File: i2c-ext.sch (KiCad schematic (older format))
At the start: 5 parts, among them J1101 SMBUS, U1101 TCA9802

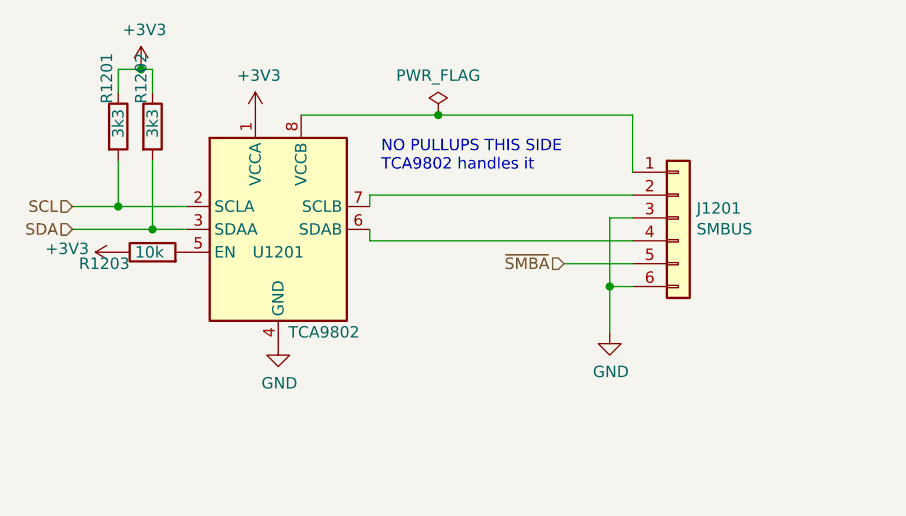
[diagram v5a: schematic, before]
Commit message: MB: add caps suggested in review
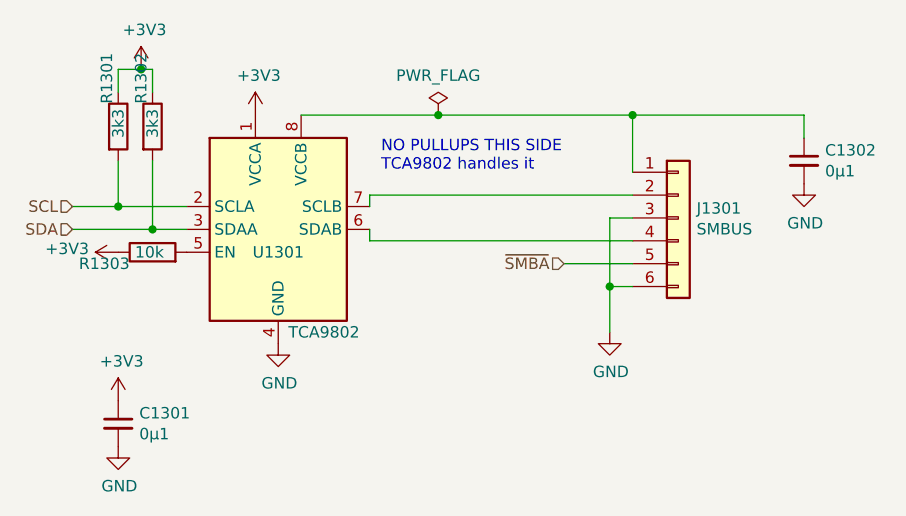
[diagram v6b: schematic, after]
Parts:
- added C1101, C1102: 0µ1, Capacitor_SMD:C_0603_1608Metric, symbol Device:C_Small
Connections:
- net +3V3: now also C1101.1
- net GND: now also C1101.2, C1102.2
- net at J1101.1 (Pin_1), U1101.8 (VCCB): now also C1102.1
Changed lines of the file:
@@
 $Descr A4 11693 8268
 encoding utf-8
-Sheet 12 15
+Sheet 13 15
 Title "Offboard I2C connector (one bus)"
 Date ""
@@
 AR Path="/5F2FE5B6/5F2F1DD6" Ref="U1201"  Part="1"
 AR Path="/5F3042B8/5F2F1DD6" Ref="U1301"  Part="1"
-F 0 "U1201" H 5600 3550 50  0000 C CNN
+F 0 "U1301" H 5600 3550 50  0000 C CNN
 F 1 "TCA9802" H 5800 3200 50  0000 C CNN
 F 2 "Package_SO:VSSOP-8_3.0x3.0mm_P0.65mm" H 6500 3200 50  0001 C CNN
@@
 AR Path="/5F2FE5B6/5F2F21C9" Ref="#PWR01203"  Part="1"
 AR Path="/5F3042B8/5F2F21C9" Ref="#PWR01303"  Part="1"
-F 0 "#PWR01203" H 5500 3000 50  0001 C CNN
+F 0 "#PWR01303" H 5500 3000 50  0001 C CNN
 F 1 "+3V3" H 5515 3323 50  0000 C CNN
 F 2 "" H 5500 3150 50  0001 C CNN
@@
 AR Path="/5F2FE5B6/5F2F2367" Ref="#PWR01204"  Part="1"
 AR Path="/5F3042B8/5F2F2367" Ref="#PWR01304"  Part="1"
-F 0 "#PWR01204" H 5600 3900 50  0001 C CNN
+F 0 "#PWR01304" H 5600 3900 50  0001 C CNN
 F 1 "GND" H 5605 3977 50  0000 C CNN
 F 2 "" H 5600 4150 50  0001 C CNN
@@
 AR Path="/5F2FE5B6/5F2F26BC" Ref="J1201"  Part="1"
 AR Path="/5F3042B8/5F2F26BC" Ref="J1301"  Part="1"
-F 0 "J1201" H 7430 3642 50  0000 L CNN
+F 0 "J1301" H 7430 3642 50  0000 L CNN
 F 1 "SMBUS" H 7430 3551 50  0000 L CNN
 F 2 "molex-sl:SL_1x06_Vertical_SMD" H 7350 3600 50  0001 C CNN
@@
 AR Path="/5F2FE5B6/5F2F3249" Ref="#PWR01205"  Part="1"
 AR Path="/5F3042B8/5F2F3249" Ref="#PWR01305"  Part="1"
-F 0 "#PWR01205" H 7050 3850 50  0001 C CNN
+F 0 "#PWR01305" H 7050 3850 50  0001 C CNN
 F 1 "GND" H 7055 3927 50  0000 C CNN
 F 2 "" H 7050 4100 50  0001 C CNN
@@
 AR Path="/5F2FE5B6/5F2F4AED" Ref="R1201"  Part="1"
 AR Path="/5F3042B8/5F2F4AED" Ref="R1301"  Part="1"
-F 0 "R1201" V 4850 3300 50  0000 L CNN
+F 0 "R1301" V 4850 3300 50  0000 L CNN
 F 1 "3k3" V 4900 3150 50  0000 L CNN
 F 2 "Resistor_SMD:R_0603_1608Metric" V 4830 3200 50  0001 C CNN
@@
 AR Path="/5F2FE5B6/5F2F511D" Ref="R1202"  Part="1"
 AR Path="/5F3042B8/5F2F511D" Ref="R1302"  Part="1"
-F 0 "R1202" V 5000 3300 50  0000 L CNN
+F 0 "R1302" V 5000 3300 50  0000 L CNN
 F 1 "3k3" V 5050 3150 50  0000 L CNN
 F 2 "Resistor_SMD:R_0603_1608Metric" V 4980 3200 50  0001 C CNN
@@
 AR Path="/5F2FE5B6/5F2F5A4A" Ref="#PWR01202"  Part="1"
 AR Path="/5F3042B8/5F2F5A4A" Ref="#PWR01302"  Part="1"
-F 0 "#PWR01202" H 5000 2800 50  0001 C CNN
+F 0 "#PWR01302" H 5000 2800 50  0001 C CNN
 F 1 "+3V3" H 5015 3123 50  0000 C CNN
 F 2 "" H 5000 2950 50  0001 C CNN
@@
 AR Path="/5F2FE5B6/600BC5DC" Ref="R1203"  Part="1"
 AR Path="/5F3042B8/600BC5DC" Ref="R1303"  Part="1"
-F 0 "R1203" V 5000 3850 50  0000 L CNN
+F 0 "R1303" V 5000 3850 50  0000 L CNN
 F 1 "10k" V 5050 3700 50  0000 L CNN
 F 2 "Resistor_SMD:R_0603_1608Metric" V 4980 3750 50  0001 C CNN
@@
 AR Path="/5F2FE5B6/600BD49C" Ref="#PWR01201"  Part="1"
 AR Path="/5F3042B8/600BD49C" Ref="#PWR01301"  Part="1"
-F 0 "#PWR01201" H 4900 3600 50  0001 C CNN
+F 0 "#PWR01301" H 4900 3600 50  0001 C CNN
 F 1 "+3V3" V 4915 3878 50  0000 L CNN
 F 2 "" H 4900 3750 50  0001 C CNN
@@
 AR Path="/5F2FE5B6/60108223" Ref="#FLG01201"  Part="1"
 AR Path="/5F3042B8/60108223" Ref="#FLG01301"  Part="1"
-F 0 "#FLG01201" H 6300 3225 50  0001 C CNN
+F 0 "#FLG01301" H 6300 3225 50  0001 C CNN
 F 1 "PWR_FLAG" H 6300 3323 50  0000 C CNN
 F 2 "" H 6300 3150 50  0001 C CNN
@@
 Wire Wire Line
 	7050 3900 7050 4100
+$Comp
+L Device:C_Small C?
+U 1 1 5F6C7B85
+P 7900 3350
+AR Path="/5F1928E5/5F29584B/5F6C7B85" Ref="C?"  Part="1"
+AR Path="/5F2F1B47/5F6C7B85" Ref="C1102"  Part="1"
+AR Path="/5F2FE5B6/5F6C7B85" Ref="C1202"  Part="1"
+AR Path="/5F3042B8/5F6C7B85" Ref="C1302"  Part="1"
+F 0 "C1302" H 7992 3396 50  0000 L CNN
+F 1 "0µ1" H 7992 3305 50  0000 L CNN
+F 2 "Capacitor_SMD:C_0603_1608Metric" H 7900 3350 50  0001 C CNN
+F 3 "~" H 7900 3350 50  0001 C CNN
+F 4 "CL10B104KB8NNWC" H 7900 3350 50  0001 C CNN "Mfg Part Num"
+F 5 "Samsung Electro-Mechanics" H 7900 3350 50  0001 C CNN "Mfg"
+	1    7900 3350
+	1    0    0    -1
+$EndComp
+Wire Wire Line
+	7150 3150 7900 3150
+Wire Wire Line
+	7900 3150 7900 3250
+Connection ~ 7150 3150
+$Comp
+L power:GND #PWR01108
+U 1 1 5F6C815F
+P 7900 3450
+AR Path="/5F2F1B47/5F6C815F" Ref="#PWR01108"  Part="1"
+AR Path="/5F2F7878/5F6C815F" Ref="#PWR?"  Part="1"
+AR Path="/5F2FE5B6/5F6C815F" Ref="#PWR01208"  Part="1"
+AR Path="/5F3042B8/5F6C815F" Ref="#PWR01308"  Part="1"
+F 0 "#PWR01308" H 7900 3200 50  0001 C CNN
+F 1 "GND" H 7905 3277 50  0000 C CNN
+F 2 "" H 7900 3450 50  0001 C CNN
+F 3 "" H 7900 3450 50  0001 C CNN
+	1    7900 3450
+	1    0    0    -1
+$EndComp
+$Comp
+L Device:C_Small C?
+U 1 1 5F6C8975
+P 4900 4500
+AR Path="/5F1928E5/5F29584B/5F6C8975" Ref="C?"  Part="1"
+AR Path="/5F2F1B47/5F6C8975" Ref="C1101"  Part="1"
+AR Path="/5F2FE5B6/5F6C8975" Ref="C1201"  Part="1"
+AR Path="/5F3042B8/5F6C8975" Ref="C1301"  Part="1"
+F 0 "C1301" H 4992 4546 50  0000 L CNN
+F 1 "0µ1" H 4992 4455 50  0000 L CNN
+F 2 "Capacitor_SMD:C_0603_1608Metric" H 4900 4500 50  0001 C CNN
+F 3 "~" H 4900 4500 50  0001 C CNN
+F 4 "CL10B104KB8NNWC" H 4900 4500 50  0001 C CNN "Mfg Part Num"
+F 5 "Samsung Electro-Mechanics" H 4900 4500 50  0001 C CNN "Mfg"
+	1    4900 4500
+	1    0    0    -1
+$EndComp
+$Comp
+L power:+3V3 #PWR01106
+U 1 1 5F6C8BE6
+P 4900 4400
+AR Path="/5F2F1B47/5F6C8BE6" Ref="#PWR01106"  Part="1"
+AR Path="/5F2F7878/5F6C8BE6" Ref="#PWR?"  Part="1"
+AR Path="/5F2FE5B6/5F6C8BE6" Ref="#PWR01206"  Part="1"
+AR Path="/5F3042B8/5F6C8BE6" Ref="#PWR01306"  Part="1"
+F 0 "#PWR01306" H 4900 4250 50  0001 C CNN
+F 1 "+3V3" H 4915 4573 50  0000 C CNN
+F 2 "" H 4900 4400 50  0001 C CNN
+F 3 "" H 4900 4400 50  0001 C CNN
+	1    4900 4400
+	1    0    0    -1
+$EndComp
+$Comp
+L power:GND #PWR01107
+U 1 1 5F6C90F3
+P 4900 4600
+AR Path="/5F2F1B47/5F6C90F3" Ref="#PWR01107"  Part="1"
+AR Path="/5F2F7878/5F6C90F3" Ref="#PWR?"  Part="1"
+AR Path="/5F2FE5B6/5F6C90F3" Ref="#PWR01207"  Part="1"
+AR Path="/5F3042B8/5F6C90F3" Ref="#PWR01307"  Part="1"
+F 0 "#PWR01307" H 4900 4350 50  0001 C CNN
+F 1 "GND" H 4905 4427 50  0000 C CNN
+F 2 "" H 4900 4600 50  0001 C CNN
+F 3 "" H 4900 4600 50  0001 C CNN
+	1    4900 4600
+	1    0    0    -1
+$EndComp
 $EndSCHEMATC

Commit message: Update MPNs to full, orderable, normally-stocked MPNs
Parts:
- U1101: Mfg Part Num TCA9802 -> TCA9802DGKR
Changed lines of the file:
@@
 F 3 "http://www.ti.com/lit/ds/symlink/tca9802.pdf" H 5300 4100 50  0001 C CNN
 F 4 "Texas Instruments" H 5600 3650 50  0001 C CNN "Mfg"
-F 5 "TCA9802" H 5600 3650 50  0001 C CNN "Mfg Part Num"
+F 5 "TCA9802DGKR" H 5600 3650 50  0001 C CNN "Mfg Part Num"
 	1    5600 3650
 	1    0    0    -1

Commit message: gemini-bringup: Add CPNs for all components
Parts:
- C1101, C1102: CPN (none) -> 212-00011
- J1101: CPN (none) -> 215-00028
- R1101, R1102: CPN (none) -> 232-00018
- R1103: CPN (none) -> 232-00024
- U1101: CPN (none) -> 221-00022
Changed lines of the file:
@@
 F 4 "Texas Instruments" H 5600 3650 50  0001 C CNN "Mfg"
 F 5 "TCA9802DGKR" H 5600 3650 50  0001 C CNN "Mfg Part Num"
+F 6 "221-00022" H 5600 3650 50  0001 C CNN "CPN"
 	1    5600 3650
 	1    0    0    -1
@@
 F 4 "Molex" H 7350 3600 50  0001 C CNN "Mfg"
 F 5 "0740991006" H 7350 3600 50  0001 C CNN "Mfg Part Num"
+F 6 "215-00028" H 7350 3600 50  0001 C CNN "CPN"
 	1    7350 3600
 	1    0    0    -1
@@
 F 4 "CR0603-JW-332ELF" H 4900 3200 50  0001 C CNN "Mfg Part Num"
 F 5 "Bourns" H 4900 3200 50  0001 C CNN "Mfg"
+F 6 "232-00018" H 4900 3200 50  0001 C CNN "CPN"
 	1    4900 3200
 	1    0    0    -1
@@
 F 4 "CR0603-JW-332ELF" H 5050 3200 50  0001 C CNN "Mfg Part Num"
 F 5 "Bourns" H 5050 3200 50  0001 C CNN "Mfg"
+F 6 "232-00018" H 5050 3200 50  0001 C CNN "CPN"
 	1    5050 3200
 	1    0    0    -1
@@
 F 4 "CR0603-JW-103ELF" H 5050 3750 50  0001 C CNN "Mfg Part Num"
 F 5 "Bourns" H 5050 3750 50  0001 C CNN "Mfg"
+F 6 "232-00024" H 5050 3750 50  0001 C CNN "CPN"
 	1    5050 3750
 	0    -1   -1   0
@@
 F 4 "CL10B104KB8NNWC" H 7900 3350 50  0001 C CNN "Mfg Part Num"
 F 5 "Samsung Electro-Mechanics" H 7900 3350 50  0001 C CNN "Mfg"
+F 6 "212-00011" H 7900 3350 50  0001 C CNN "CPN"
 	1    7900 3350
 	1    0    0    -1
@@
 F 4 "CL10B104KB8NNWC" H 4900 4500 50  0001 C CNN "Mfg Part Num"
 F 5 "Samsung Electro-Mechanics" H 4900 4500 50  0001 C CNN "Mfg"
+F 6 "212-00011" H 4900 4500 50  0001 C CNN "CPN"
 	1    4900 4500
 	1    0    0    -1
